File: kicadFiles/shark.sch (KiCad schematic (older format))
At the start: 258 parts, among them J1 USB_C_Receptacle, Q1 AO4406AL, SW1 MXSwitch, SW10 MXSwitch, SW11 MXSwitch, SW12 MXSwitch, SW13 MXSwitch, SW14 MXSwitch, SW15 MXSwitch, SW16 MXSwitch, SW17 MXSwitch, SW18 MXSwitch, SW19 MXSwitch, SW2 MXSwitch, SW20 MXSwitch, SW21 MXSwitch, SW22 MXSwitch, SW23 MXSwitch, SW24 MXSwitch, SW25 MXSwitch, SW26 MXSwitch, SW27 MXSwitch, SW28 MXSwitch, SW29 MXSwitch, SW3 MXSwitch, SW30 MXSwitch, SW31 MXSwitch, SW32 MXSwitch, SW33 MXSwitch, SW34 MXSwitch, SW35 MXSwitch, SW36 MXSwitch, SW37 MXSwitch, SW38 MXSwitch, SW39 MXSwitch, SW4 MXSwitch, SW40 MXSwitch, SW41 MXSwitch, SW42 MXSwitch, SW43 MXSwitch, SW44 MXSwitch, SW45 MXSwitch, SW46 MXSwitch, SW47 MXSwitch, SW48 MXSwitch, SW49 MXSwitch, SW5 MXSwitch, SW50 MXSwitch, SW51 MXSwitch, SW6 MXSwitch, SW7 MXSwitch, SW8 MXSwitch, SW9 MXSwitch, U1 STM32F303CCT7, U2 MCP1700-3302E_SOT23, Y1 8MHz

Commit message: Reorganized folders
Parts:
- D1, D48: footprint Keyboard_switches:D_SOD-123 -> acheronSymbols:D_SOD-123
- D10: renamed from D15; footprint Keyboard_switches:D_SOD-123 -> acheronSymbols:D_SOD-123
- D11: renamed from D27; footprint Keyboard_switches:D_SOD-123 -> acheronSymbols:D_SOD-123
- D12: renamed from D39; footprint Keyboard_switches:D_SOD-123 -> acheronSymbols:D_SOD-123
- D13: renamed from D4; footprint Keyboard_switches:D_SOD-123 -> acheronSymbols:D_SOD-123
- D14: renamed from D16; footprint Keyboard_switches:D_SOD-123 -> acheronSymbols:D_SOD-123
- D15: renamed from D28; footprint Keyboard_switches:D_SOD-123 -> acheronSymbols:D_SOD-123
- D16: renamed from D40; footprint Keyboard_switches:D_SOD-123 -> acheronSymbols:D_SOD-123
- D17: renamed from D5; footprint Keyboard_switches:D_SOD-123 -> acheronSymbols:D_SOD-123
- D18: renamed from D17; footprint Keyboard_switches:D_SOD-123 -> acheronSymbols:D_SOD-123
- D19: renamed from D29; footprint Keyboard_switches:D_SOD-123 -> acheronSymbols:D_SOD-123
- D2: renamed from D13; footprint Keyboard_switches:D_SOD-123 -> acheronSymbols:D_SOD-123
- D20: renamed from D41; footprint Keyboard_switches:D_SOD-123 -> acheronSymbols:D_SOD-123
- D21: renamed from D6; footprint Keyboard_switches:D_SOD-123 -> acheronSymbols:D_SOD-123
- D22: renamed from D18; footprint Keyboard_switches:D_SOD-123 -> acheronSymbols:D_SOD-123
- D23: renamed from D30; footprint Keyboard_switches:D_SOD-123 -> acheronSymbols:D_SOD-123
- D24: renamed from D42; footprint Keyboard_switches:D_SOD-123 -> acheronSymbols:D_SOD-123
- D25: renamed from D7; footprint Keyboard_switches:D_SOD-123 -> acheronSymbols:D_SOD-123
- D26: renamed from D19; footprint Keyboard_switches:D_SOD-123 -> acheronSymbols:D_SOD-123
- D27: renamed from D31; footprint Keyboard_switches:D_SOD-123 -> acheronSymbols:D_SOD-123
- D28: renamed from D43; footprint Keyboard_switches:D_SOD-123 -> acheronSymbols:D_SOD-123
- D29: renamed from D8; footprint Keyboard_switches:D_SOD-123 -> acheronSymbols:D_SOD-123
- D3: renamed from D25; footprint Keyboard_switches:D_SOD-123 -> acheronSymbols:D_SOD-123
- D30: renamed from D20; footprint Keyboard_switches:D_SOD-123 -> acheronSymbols:D_SOD-123
- D31: renamed from D32; footprint Keyboard_switches:D_SOD-123 -> acheronSymbols:D_SOD-123
- D32: renamed from D44; footprint Keyboard_switches:D_SOD-123 -> acheronSymbols:D_SOD-123
- D33: renamed from D9; footprint Keyboard_switches:D_SOD-123 -> acheronSymbols:D_SOD-123
- D34: renamed from D21; footprint Keyboard_switches:D_SOD-123 -> acheronSymbols:D_SOD-123
- D35: renamed from D33; footprint Keyboard_switches:D_SOD-123 -> acheronSymbols:D_SOD-123
- D36: renamed from D45; footprint Keyboard_switches:D_SOD-123 -> acheronSymbols:D_SOD-123
- D37: renamed from D10; footprint Keyboard_switches:D_SOD-123 -> acheronSymbols:D_SOD-123
- D38: renamed from D22; footprint Keyboard_switches:D_SOD-123 -> acheronSymbols:D_SOD-123
- D39: renamed from D34; footprint Keyboard_switches:D_SOD-123 -> acheronSymbols:D_SOD-123
- D4: renamed from D37; footprint Keyboard_switches:D_SOD-123 -> acheronSymbols:D_SOD-123
- D40: renamed from D46; footprint Keyboard_switches:D_SOD-123 -> acheronSymbols:D_SOD-123
- D41: renamed from D11; footprint Keyboard_switches:D_SOD-123 -> acheronSymbols:D_SOD-123
- D42: renamed from D23; footprint Keyboard_switches:D_SOD-123 -> acheronSymbols:D_SOD-123
- D43: renamed from D35; footprint Keyboard_switches:D_SOD-123 -> acheronSymbols:D_SOD-123
- D44: renamed from D47; footprint Keyboard_switches:D_SOD-123 -> acheronSymbols:D_SOD-123
- D45: renamed from D12; footprint Keyboard_switches:D_SOD-123 -> acheronSymbols:D_SOD-123
- D46: renamed from D24; footprint Keyboard_switches:D_SOD-123 -> acheronSymbols:D_SOD-123
- D47: renamed from D36; footprint Keyboard_switches:D_SOD-123 -> acheronSymbols:D_SOD-123
- D5: renamed from D2; footprint Keyboard_switches:D_SOD-123 -> acheronSymbols:D_SOD-123
- D6: renamed from D14; footprint Keyboard_switches:D_SOD-123 -> acheronSymbols:D_SOD-123
- D7: renamed from D26; footprint Keyboard_switches:D_SOD-123 -> acheronSymbols:D_SOD-123
- D8: renamed from D38; footprint Keyboard_switches:D_SOD-123 -> acheronSymbols:D_SOD-123
- D9: renamed from D3; footprint Keyboard_switches:D_SOD-123 -> acheronSymbols:D_SOD-123
- LED1, LED47: footprint Keyboard_switches:thtLED -> acheronSymbols:thtLED; symbol Keyboard_switches:LED -> acheronSymbols:LED
- LED10: renamed from LED15; footprint Keyboard_switches:thtLED -> acheronSymbols:thtLED; symbol Keyboard_switches:LED -> acheronSymbols:LED
- LED11: renamed from LED27; footprint Keyboard_switches:thtLED -> acheronSymbols:thtLED; symbol Keyboard_switches:LED -> acheronSymbols:LED
- LED12: renamed from LED39; footprint Keyboard_switches:thtLED -> acheronSymbols:thtLED; symbol Keyboard_switches:LED -> acheronSymbols:LED
- LED13: renamed from LED4; footprint Keyboard_switches:thtLED -> acheronSymbols:thtLED; symbol Keyboard_switches:LED -> acheronSymbols:LED
- LED14: renamed from LED16; footprint Keyboard_switches:thtLED -> acheronSymbols:thtLED; symbol Keyboard_switches:LED -> acheronSymbols:LED
- LED15: renamed from LED28; footprint Keyboard_switches:thtLED -> acheronSymbols:thtLED; symbol Keyboard_switches:LED -> acheronSymbols:LED
- LED16: renamed from LED40; footprint Keyboard_switches:thtLED -> acheronSymbols:thtLED; symbol Keyboard_switches:LED -> acheronSymbols:LED
- LED17: renamed from LED5; footprint Keyboard_switches:thtLED -> acheronSymbols:thtLED; symbol Keyboard_switches:LED -> acheronSymbols:LED
- LED18: renamed from LED17; footprint Keyboard_switches:thtLED -> acheronSymbols:thtLED; symbol Keyboard_switches:LED -> acheronSymbols:LED
- LED19: renamed from LED29; footprint Keyboard_switches:thtLED -> acheronSymbols:thtLED; symbol Keyboard_switches:LED -> acheronSymbols:LED
- LED2: renamed from LED13; footprint Keyboard_switches:thtLED -> acheronSymbols:thtLED; symbol Keyboard_switches:LED -> acheronSymbols:LED
- LED20: renamed from LED41; footprint Keyboard_switches:thtLED -> acheronSymbols:thtLED; symbol Keyboard_switches:LED -> acheronSymbols:LED
- LED21: renamed from LED49; footprint Keyboard_switches:thtLED -> acheronSymbols:thtLED; symbol Keyboard_switches:LED -> acheronSymbols:LED
- LED22: renamed from LED6; footprint Keyboard_switches:thtLED -> acheronSymbols:thtLED; symbol Keyboard_switches:LED -> acheronSymbols:LED
- LED23: renamed from LED18; footprint Keyboard_switches:thtLED -> acheronSymbols:thtLED; symbol Keyboard_switches:LED -> acheronSymbols:LED
- LED24: renamed from LED30; footprint Keyboard_switches:thtLED -> acheronSymbols:thtLED; symbol Keyboard_switches:LED -> acheronSymbols:LED
- LED25: renamed from LED42; footprint Keyboard_switches:thtLED -> acheronSymbols:thtLED; symbol Keyboard_switches:LED -> acheronSymbols:LED
- LED26: renamed from LED50; footprint Keyboard_switches:thtLED -> acheronSymbols:thtLED; symbol Keyboard_switches:LED -> acheronSymbols:LED
- LED27: renamed from LED7; footprint Keyboard_switches:thtLED -> acheronSymbols:thtLED; symbol Keyboard_switches:LED -> acheronSymbols:LED
- LED28: renamed from LED19; footprint Keyboard_switches:thtLED -> acheronSymbols:thtLED; symbol Keyboard_switches:LED -> acheronSymbols:LED
- LED29: renamed from LED31; footprint Keyboard_switches:thtLED -> acheronSymbols:thtLED; symbol Keyboard_switches:LED -> acheronSymbols:LED
- LED3: renamed from LED25; footprint Keyboard_switches:thtLED -> acheronSymbols:thtLED; symbol Keyboard_switches:LED -> acheronSymbols:LED
- LED30: renamed from LED43; footprint Keyboard_switches:thtLED -> acheronSymbols:thtLED; symbol Keyboard_switches:LED -> acheronSymbols:LED
- LED31: renamed from LED51; footprint Keyboard_switches:thtLED -> acheronSymbols:thtLED; symbol Keyboard_switches:LED -> acheronSymbols:LED
- LED32: renamed from LED8; footprint Keyboard_switches:thtLED -> acheronSymbols:thtLED; symbol Keyboard_switches:LED -> acheronSymbols:LED
- LED33: renamed from LED20; footprint Keyboard_switches:thtLED -> acheronSymbols:thtLED; symbol Keyboard_switches:LED -> acheronSymbols:LED
- LED34: renamed from LED32; footprint Keyboard_switches:thtLED -> acheronSymbols:thtLED; symbol Keyboard_switches:LED -> acheronSymbols:LED
- LED35: renamed from LED44; footprint Keyboard_switches:thtLED -> acheronSymbols:thtLED; symbol Keyboard_switches:LED -> acheronSymbols:LED
- LED36: renamed from LED9; footprint Keyboard_switches:thtLED -> acheronSymbols:thtLED; symbol Keyboard_switches:LED -> acheronSymbols:LED
- LED37: renamed from LED21; footprint Keyboard_switches:thtLED -> acheronSymbols:thtLED; symbol Keyboard_switches:LED -> acheronSymbols:LED
- LED38: renamed from LED33; footprint Keyboard_switches:thtLED -> acheronSymbols:thtLED; symbol Keyboard_switches:LED -> acheronSymbols:LED
- LED39: renamed from LED45; footprint Keyboard_switches:thtLED -> acheronSymbols:thtLED; symbol Keyboard_switches:LED -> acheronSymbols:LED
- LED4: renamed from LED37; footprint Keyboard_switches:thtLED -> acheronSymbols:thtLED; symbol Keyboard_switches:LED -> acheronSymbols:LED
- LED40: renamed from LED10; footprint Keyboard_switches:thtLED -> acheronSymbols:thtLED; symbol Keyboard_switches:LED -> acheronSymbols:LED
- LED41: renamed from LED22; footprint Keyboard_switches:thtLED -> acheronSymbols:thtLED; symbol Keyboard_switches:LED -> acheronSymbols:LED
- LED42: renamed from LED34; footprint Keyboard_switches:thtLED -> acheronSymbols:thtLED; symbol Keyboard_switches:LED -> acheronSymbols:LED
- LED43: renamed from LED46; footprint Keyboard_switches:thtLED -> acheronSymbols:thtLED; symbol Keyboard_switches:LED -> acheronSymbols:LED
- LED44: renamed from LED11; footprint Keyboard_switches:thtLED -> acheronSymbols:thtLED; symbol Keyboard_switches:LED -> acheronSymbols:LED
- LED45: renamed from LED23; footprint Keyboard_switches:thtLED -> acheronSymbols:thtLED; symbol Keyboard_switches:LED -> acheronSymbols:LED
- LED46: renamed from LED35; footprint Keyboard_switches:thtLED -> acheronSymbols:thtLED; symbol Keyboard_switches:LED -> acheronSymbols:LED
- LED48: renamed from LED12; footprint Keyboard_switches:thtLED -> acheronSymbols:thtLED; symbol Keyboard_switches:LED -> acheronSymbols:LED
- LED49: renamed from LED24; footprint Keyboard_switches:thtLED -> acheronSymbols:thtLED; symbol Keyboard_switches:LED -> acheronSymbols:LED
- LED5: renamed from LED2; footprint Keyboard_switches:thtLED -> acheronSymbols:thtLED; symbol Keyboard_switches:LED -> acheronSymbols:LED
- LED50: renamed from LED36; footprint Keyboard_switches:thtLED -> acheronSymbols:thtLED; symbol Keyboard_switches:LED -> acheronSymbols:LED
- LED51: renamed from LED48; footprint Keyboard_switches:thtLED -> acheronSymbols:thtLED; symbol Keyboard_switches:LED -> acheronSymbols:LED
- LED6: renamed from LED14; footprint Keyboard_switches:thtLED -> acheronSymbols:thtLED; symbol Keyboard_switches:LED -> acheronSymbols:LED
- LED7: renamed from LED26; footprint Keyboard_switches:thtLED -> acheronSymbols:thtLED; symbol Keyboard_switches:LED -> acheronSymbols:LED
- LED8: renamed from LED38; footprint Keyboard_switches:thtLED -> acheronSymbols:thtLED; symbol Keyboard_switches:LED -> acheronSymbols:LED
- LED9: renamed from LED3; footprint Keyboard_switches:thtLED -> acheronSymbols:thtLED; symbol Keyboard_switches:LED -> acheronSymbols:LED
- Q1: footprint Keyboard_switches:AO4406AL -> acheronSymbols:AO4406AL; symbol Keyboard_switches:AO4406AL -> acheronSymbols:AO4406AL
- RGB1, RGB8: footprint Keyboard_switches:LED_WS2812B -> acheronSymbols:LED_WS2812B
- RGB2: renamed from RGB5; footprint Keyboard_switches:LED_WS2812B -> acheronSymbols:LED_WS2812B
- RGB3: renamed from RGB2; footprint Keyboard_switches:LED_WS2812B -> acheronSymbols:LED_WS2812B
- RGB4: renamed from RGB6; footprint Keyboard_switches:LED_WS2812B -> acheronSymbols:LED_WS2812B
- RGB5: renamed from RGB3; footprint Keyboard_switches:LED_WS2812B -> acheronSymbols:LED_WS2812B
- RGB6: renamed from RGB7; footprint Keyboard_switches:LED_WS2812B -> acheronSymbols:LED_WS2812B
- RGB7: renamed from RGB4; footprint Keyboard_switches:LED_WS2812B -> acheronSymbols:LED_WS2812B
- SW1, SW47: footprint Keyboard_switches:MX100 -> acheronSymbols:MX100; symbol Keyboard_switches:MXSwitch -> acheronSymbols:MXSwitch
- SW10: renamed from SW15; footprint Keyboard_switches:MX100 -> acheronSymbols:MX100; symbol Keyboard_switches:MXSwitch -> acheronSymbols:MXSwitch
- SW11: renamed from SW27; footprint Keyboard_switches:MX100 -> acheronSymbols:MX100; symbol Keyboard_switches:MXSwitch -> acheronSymbols:MXSwitch
- SW12: renamed from SW39; footprint Keyboard_switches:MX100 -> acheronSymbols:MX100; symbol Keyboard_switches:MXSwitch -> acheronSymbols:MXSwitch
- SW13: renamed from SW4; footprint Keyboard_switches:MX100 -> acheronSymbols:MX100; symbol Keyboard_switches:MXSwitch -> acheronSymbols:MXSwitch
- SW14: renamed from SW16; footprint Keyboard_switches:MX100 -> acheronSymbols:MX100; symbol Keyboard_switches:MXSwitch -> acheronSymbols:MXSwitch
- SW15: renamed from SW28; footprint Keyboard_switches:MX100 -> acheronSymbols:MX100; symbol Keyboard_switches:MXSwitch -> acheronSymbols:MXSwitch
- SW16: renamed from SW40; footprint Keyboard_switches:MX100 -> acheronSymbols:MX100; symbol Keyboard_switches:MXSwitch -> acheronSymbols:MXSwitch
- SW17: renamed from SW5; footprint Keyboard_switches:MX100 -> acheronSymbols:MX100; symbol Keyboard_switches:MXSwitch -> acheronSymbols:MXSwitch
- SW18: renamed from SW17; footprint Keyboard_switches:MX100 -> acheronSymbols:MX100; symbol Keyboard_switches:MXSwitch -> acheronSymbols:MXSwitch
- SW19: renamed from SW29; footprint Keyboard_switches:MX100 -> acheronSymbols:MX100; symbol Keyboard_switches:MXSwitch -> acheronSymbols:MXSwitch
- SW2: renamed from SW13; footprint Keyboard_switches:MX100 -> acheronSymbols:MX100; symbol Keyboard_switches:MXSwitch -> acheronSymbols:MXSwitch
- SW20: renamed from SW41; footprint Keyboard_switches:MX100 -> acheronSymbols:MX100; symbol Keyboard_switches:MXSwitch -> acheronSymbols:MXSwitch
- SW21: renamed from SW49; footprint Keyboard_switches:MX200R -> acheronSymbols:MX200R; symbol Keyboard_switches:MXSwitch -> acheronSymbols:MXSwitch
- SW22: renamed from SW6; footprint Keyboard_switches:MX100 -> acheronSymbols:MX100; symbol Keyboard_switches:MXSwitch -> acheronSymbols:MXSwitch
- SW23: renamed from SW18; footprint Keyboard_switches:MX100 -> acheronSymbols:MX100; symbol Keyboard_switches:MXSwitch -> acheronSymbols:MXSwitch
- SW24: renamed from SW30; footprint Keyboard_switches:MX100 -> acheronSymbols:MX100; symbol Keyboard_switches:MXSwitch -> acheronSymbols:MXSwitch
- SW25: renamed from SW42; footprint Keyboard_switches:MX100 -> acheronSymbols:MX100; symbol Keyboard_switches:MXSwitch -> acheronSymbols:MXSwitch
- renumbered C9 to C1, C7 to C2, C1 to C3, C2 to C4, CSRT2 to CSRT1, H12 to H1, H1 to H2, H2 to H3, H3 to H4, H4 to H5, H5 to H6, H6 to H7, R6 to R1, R5 to R2, RA2 to RA1, RA1 to RA2, RB2 to RB1, RB1 to RB2, RL15 to RL10, RL27 to RL11, RL39 to RL12, RL4 to RL13, RL16 to RL14, RL28 to RL15, RL40 to RL16, RL5 to RL17, RL17 to RL18, RL29 to RL19, RL13 to RL2, RL41 to RL20, RL6 to RL21, RL18 to RL22, RL30 to RL23, RL42 to RL24, RL7 to RL25, RL19 to RL26, RL31 to RL27, RL43 to RL28, RL8 to RL29, RL25 to RL3, RL20 to RL30, RL32 to RL31, RL44 to RL32, RL9 to RL33, RL21 to RL34, RL33 to RL35, RL45 to RL36, RL10 to RL37, RL22 to RL38, RL34 to RL39, RL37 to RL4, RL46 to RL40, RL11 to RL41, RL23 to RL42, RL35 to RL43, RL47 to RL44, RL12 to RL45, RL24 to RL46, RL36 to RL47, RL2 to RL5, RL14 to RL6, RL26 to RL7, RL38 to RL8, RL3 to RL9, U2 to U1
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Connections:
- wire segments 620 -> 573

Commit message: Added encoder position and moved push button
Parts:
- added ROT2: Rotary_Encoder_Switch, acheronHardware:ALPS_EC11E, symbol Device:Rotary_Encoder_Switch
- D1, D48: footprint acheronSymbols:D_SOD-123 -> acheronComponents:D_SOD-123
- D10: renamed from D37; footprint acheronSymbols:D_SOD-123 -> acheronComponents:D_SOD-123
- D11: renamed from D41; footprint acheronSymbols:D_SOD-123 -> acheronComponents:D_SOD-123
- D12: renamed from D45; footprint acheronSymbols:D_SOD-123 -> acheronComponents:D_SOD-123
- D13: renamed from D2; footprint acheronSymbols:D_SOD-123 -> acheronComponents:D_SOD-123
- D14: renamed from D6; footprint acheronSymbols:D_SOD-123 -> acheronComponents:D_SOD-123
- D15: renamed from D10; footprint acheronSymbols:D_SOD-123 -> acheronComponents:D_SOD-123
- D16: renamed from D14; footprint acheronSymbols:D_SOD-123 -> acheronComponents:D_SOD-123
- D17: renamed from D18; footprint acheronSymbols:D_SOD-123 -> acheronComponents:D_SOD-123
- D18: renamed from D22; footprint acheronSymbols:D_SOD-123 -> acheronComponents:D_SOD-123
- D19: renamed from D26; footprint acheronSymbols:D_SOD-123 -> acheronComponents:D_SOD-123
- D2: renamed from D5; footprint acheronSymbols:D_SOD-123 -> acheronComponents:D_SOD-123
- D20: renamed from D30; footprint acheronSymbols:D_SOD-123 -> acheronComponents:D_SOD-123
- D21: renamed from D34; footprint acheronSymbols:D_SOD-123 -> acheronComponents:D_SOD-123
- D22: renamed from D38; footprint acheronSymbols:D_SOD-123 -> acheronComponents:D_SOD-123
- D23: renamed from D42; footprint acheronSymbols:D_SOD-123 -> acheronComponents:D_SOD-123
- D24: renamed from D46; footprint acheronSymbols:D_SOD-123 -> acheronComponents:D_SOD-123
- D25: renamed from D3; footprint acheronSymbols:D_SOD-123 -> acheronComponents:D_SOD-123
- D26: renamed from D7; footprint acheronSymbols:D_SOD-123 -> acheronComponents:D_SOD-123
- D27: renamed from D11; footprint acheronSymbols:D_SOD-123 -> acheronComponents:D_SOD-123
- D28: renamed from D15; footprint acheronSymbols:D_SOD-123 -> acheronComponents:D_SOD-123
- D29: renamed from D19; footprint acheronSymbols:D_SOD-123 -> acheronComponents:D_SOD-123
- D3: renamed from D9; footprint acheronSymbols:D_SOD-123 -> acheronComponents:D_SOD-123
- D30: renamed from D23; footprint acheronSymbols:D_SOD-123 -> acheronComponents:D_SOD-123
- D31: renamed from D27; footprint acheronSymbols:D_SOD-123 -> acheronComponents:D_SOD-123
- D32: renamed from D31; footprint acheronSymbols:D_SOD-123 -> acheronComponents:D_SOD-123
- D33: renamed from D35; footprint acheronSymbols:D_SOD-123 -> acheronComponents:D_SOD-123
- D34: renamed from D39; footprint acheronSymbols:D_SOD-123 -> acheronComponents:D_SOD-123
- D35: renamed from D43; footprint acheronSymbols:D_SOD-123 -> acheronComponents:D_SOD-123
- D36: renamed from D47; footprint acheronSymbols:D_SOD-123 -> acheronComponents:D_SOD-123
- D37: renamed from D4; footprint acheronSymbols:D_SOD-123 -> acheronComponents:D_SOD-123
- D38: renamed from D8; footprint acheronSymbols:D_SOD-123 -> acheronComponents:D_SOD-123
- D39: renamed from D12; footprint acheronSymbols:D_SOD-123 -> acheronComponents:D_SOD-123
- D4: renamed from D13; footprint acheronSymbols:D_SOD-123 -> acheronComponents:D_SOD-123
- D40: renamed from D16; footprint acheronSymbols:D_SOD-123 -> acheronComponents:D_SOD-123
- D41: renamed from D20; footprint acheronSymbols:D_SOD-123 -> acheronComponents:D_SOD-123
- D42: renamed from D24; footprint acheronSymbols:D_SOD-123 -> acheronComponents:D_SOD-123
- D43: renamed from D28; footprint acheronSymbols:D_SOD-123 -> acheronComponents:D_SOD-123
- D44: renamed from D32; footprint acheronSymbols:D_SOD-123 -> acheronComponents:D_SOD-123
- D45: renamed from D36; footprint acheronSymbols:D_SOD-123 -> acheronComponents:D_SOD-123
- D46: renamed from D40; footprint acheronSymbols:D_SOD-123 -> acheronComponents:D_SOD-123
- D47: renamed from D44; footprint acheronSymbols:D_SOD-123 -> acheronComponents:D_SOD-123
- D5: renamed from D17; footprint acheronSymbols:D_SOD-123 -> acheronComponents:D_SOD-123
- D6: renamed from D21; footprint acheronSymbols:D_SOD-123 -> acheronComponents:D_SOD-123
- D7: renamed from D25; footprint acheronSymbols:D_SOD-123 -> acheronComponents:D_SOD-123
- D8: renamed from D29; footprint acheronSymbols:D_SOD-123 -> acheronComponents:D_SOD-123
- D9: renamed from D33; footprint acheronSymbols:D_SOD-123 -> acheronComponents:D_SOD-123
- DF1: footprint Diode_SMD:D_SOD-123 -> acheronComponents:D_SOD-123
- LED1, LED47: footprint acheronSymbols:thtLED -> acheronComponents:thtLED
- LED10: renamed from LED40; footprint acheronSymbols:thtLED -> acheronComponents:thtLED
- LED11: renamed from LED44; footprint acheronSymbols:thtLED -> acheronComponents:thtLED
- LED12: renamed from LED48; footprint acheronSymbols:thtLED -> acheronComponents:thtLED
- LED13: renamed from LED2; footprint acheronSymbols:thtLED -> acheronComponents:thtLED
- LED14: renamed from LED6; footprint acheronSymbols:thtLED -> acheronComponents:thtLED
- LED15: renamed from LED10; footprint acheronSymbols:thtLED -> acheronComponents:thtLED
- LED16: renamed from LED14; footprint acheronSymbols:thtLED -> acheronComponents:thtLED
- LED17: renamed from LED18; footprint acheronSymbols:thtLED -> acheronComponents:thtLED
- LED18: renamed from LED23; footprint acheronSymbols:thtLED -> acheronComponents:thtLED
- LED19: renamed from LED28; footprint acheronSymbols:thtLED -> acheronComponents:thtLED
- LED2: renamed from LED5; footprint acheronSymbols:thtLED -> acheronComponents:thtLED
- LED20: renamed from LED33; footprint acheronSymbols:thtLED -> acheronComponents:thtLED
- LED21: renamed from LED37; footprint acheronSymbols:thtLED -> acheronComponents:thtLED
- LED22: renamed from LED41; footprint acheronSymbols:thtLED -> acheronComponents:thtLED
- LED23: renamed from LED45; footprint acheronSymbols:thtLED -> acheronComponents:thtLED
- LED24: renamed from LED49; footprint acheronSymbols:thtLED -> acheronComponents:thtLED
- LED25: renamed from LED3; footprint acheronSymbols:thtLED -> acheronComponents:thtLED
- LED26: renamed from LED7; footprint acheronSymbols:thtLED -> acheronComponents:thtLED
- LED27: renamed from LED11; footprint acheronSymbols:thtLED -> acheronComponents:thtLED
- LED28: renamed from LED15; footprint acheronSymbols:thtLED -> acheronComponents:thtLED
- LED29: renamed from LED19; footprint acheronSymbols:thtLED -> acheronComponents:thtLED
- LED3: renamed from LED9; footprint acheronSymbols:thtLED -> acheronComponents:thtLED
- LED30: renamed from LED24; footprint acheronSymbols:thtLED -> acheronComponents:thtLED
- LED31: renamed from LED29; footprint acheronSymbols:thtLED -> acheronComponents:thtLED
- LED32: renamed from LED34; footprint acheronSymbols:thtLED -> acheronComponents:thtLED
- LED33: renamed from LED38; footprint acheronSymbols:thtLED -> acheronComponents:thtLED
- LED34: renamed from LED42; footprint acheronSymbols:thtLED -> acheronComponents:thtLED
- LED35: renamed from LED46; footprint acheronSymbols:thtLED -> acheronComponents:thtLED
- LED36: renamed from LED50; footprint acheronSymbols:thtLED -> acheronComponents:thtLED
- LED37: renamed from LED4; footprint acheronSymbols:thtLED -> acheronComponents:thtLED
- LED38: renamed from LED8; footprint acheronSymbols:thtLED -> acheronComponents:thtLED
- LED39: renamed from LED12; footprint acheronSymbols:thtLED -> acheronComponents:thtLED
- LED4: renamed from LED13; footprint acheronSymbols:thtLED -> acheronComponents:thtLED
- LED40: renamed from LED16; footprint acheronSymbols:thtLED -> acheronComponents:thtLED
- LED41: renamed from LED20; footprint acheronSymbols:thtLED -> acheronComponents:thtLED
- LED42: renamed from LED25; footprint acheronSymbols:thtLED -> acheronComponents:thtLED
- LED43: renamed from LED30; footprint acheronSymbols:thtLED -> acheronComponents:thtLED
- LED44: renamed from LED35; footprint acheronSymbols:thtLED -> acheronComponents:thtLED
- LED45: renamed from LED39; footprint acheronSymbols:thtLED -> acheronComponents:thtLED
- LED46: renamed from LED43; footprint acheronSymbols:thtLED -> acheronComponents:thtLED
- LED48: renamed from LED51; footprint acheronSymbols:thtLED -> acheronComponents:thtLED
- LED49: renamed from LED21; footprint acheronSymbols:thtLED -> acheronComponents:thtLED
- LED5: renamed from LED17; footprint acheronSymbols:thtLED -> acheronComponents:thtLED
- LED50: renamed from LED26; footprint acheronSymbols:thtLED -> acheronComponents:thtLED
- LED51: renamed from LED31; footprint acheronSymbols:thtLED -> acheronComponents:thtLED
- LED6: renamed from LED22; footprint acheronSymbols:thtLED -> acheronComponents:thtLED
- LED7: renamed from LED27; footprint acheronSymbols:thtLED -> acheronComponents:thtLED
- LED8: renamed from LED32; footprint acheronSymbols:thtLED -> acheronComponents:thtLED
- LED9: renamed from LED36; footprint acheronSymbols:thtLED -> acheronComponents:thtLED
- Q1: footprint acheronSymbols:AO4406AL -> acheronComponents:AO4406AL
- RGB1, RGB8: footprint acheronSymbols:LED_WS2812B -> acheronComponents:LED_WS2812B
- RGB2: renamed from RGB3; footprint acheronSymbols:LED_WS2812B -> acheronComponents:LED_WS2812B
- RGB3: renamed from RGB5; footprint acheronSymbols:LED_WS2812B -> acheronComponents:LED_WS2812B
- RGB4: renamed from RGB7; footprint acheronSymbols:LED_WS2812B -> acheronComponents:LED_WS2812B
- RGB5: renamed from RGB2; footprint acheronSymbols:LED_WS2812B -> acheronComponents:LED_WS2812B
- RGB6: renamed from RGB4; footprint acheronSymbols:LED_WS2812B -> acheronComponents:LED_WS2812B
- RGB7: renamed from RGB6; footprint acheronSymbols:LED_WS2812B -> acheronComponents:LED_WS2812B
- ROT1: footprint encoders:ALPS_EC11E -> acheronHardware:ALPS_EC11E
- SW1, SW47: footprint acheronSymbols:MX100 -> acheronKeyboardSwitches:MX100
- SW10: renamed from SW40; footprint acheronSymbols:MX100 -> acheronKeyboardSwitches:MX100
- SW11: renamed from SW44; footprint acheronSymbols:MX100 -> acheronKeyboardSwitches:MX100
- SW12: renamed from SW48; footprint acheronSymbols:MX100 -> acheronKeyboardSwitches:MX100
- SW13: renamed from SW2; footprint acheronSymbols:MX100 -> acheronKeyboardSwitches:MX100
- SW14: renamed from SW6; footprint acheronSymbols:MX100 -> acheronKeyboardSwitches:MX100
- SW15: renamed from SW10; footprint acheronSymbols:MX100 -> acheronKeyboardSwitches:MX100
- SW16: renamed from SW14; footprint acheronSymbols:MX100 -> acheronKeyboardSwitches:MX100
- SW17: renamed from SW18; footprint acheronSymbols:MX100 -> acheronKeyboardSwitches:MX100
- SW18: renamed from SW23; footprint acheronSymbols:MX100 -> acheronKeyboardSwitches:MX100
- SW19: renamed from SW28; footprint acheronSymbols:MX100 -> acheronKeyboardSwitches:MX100
- SW2: renamed from SW5; footprint acheronSymbols:MX100 -> acheronKeyboardSwitches:MX100
- SW20: renamed from SW33; footprint acheronSymbols:MX100 -> acheronKeyboardSwitches:MX100
- SW21: renamed from SW37; footprint acheronSymbols:MX100 -> acheronKeyboardSwitches:MX100
- SW22: renamed from SW41; footprint acheronSymbols:MX100 -> acheronKeyboardSwitches:MX100
- SW23: renamed from SW45; footprint acheronSymbols:MX100 -> acheronKeyboardSwitches:MX100
- SW24: renamed from SW49; footprint acheronSymbols:MX100 -> acheronKeyboardSwitches:MX100
- SW25: renamed from SW3; footprint acheronSymbols:MX100 -> acheronKeyboardSwitches:MX100
- SW26: renamed from SW7; footprint acheronSymbols:MX100 -> acheronKeyboardSwitches:MX100
- SW27: renamed from SW11; footprint acheronSymbols:MX100 -> acheronKeyboardSwitches:MX100
- SW28: renamed from SW15; footprint acheronSymbols:MX100 -> acheronKeyboardSwitches:MX100
- SW29: renamed from SW19; footprint acheronSymbols:MX100 -> acheronKeyboardSwitches:MX100
- SW3: renamed from SW9; footprint acheronSymbols:MX100 -> acheronKeyboardSwitches:MX100
- SW30: renamed from SW24; footprint acheronSymbols:MX100 -> acheronKeyboardSwitches:MX100
- SW31: renamed from SW29; footprint acheronSymbols:MX100 -> acheronKeyboardSwitches:MX100
- SW32: renamed from SW34; footprint acheronSymbols:MX100 -> acheronKeyboardSwitches:MX100
- SW33: renamed from SW38; footprint acheronSymbols:MX100 -> acheronKeyboardSwitches:MX100
- SW34: renamed from SW42; footprint acheronSymbols:MX100 -> acheronKeyboardSwitches:MX100
- SW35: renamed from SW46; footprint acheronSymbols:MX100 -> acheronKeyboardSwitches:MX100
- SW36: renamed from SW50; footprint acheronSymbols:MX100 -> acheronKeyboardSwitches:MX100
- SW37: renamed from SW4; footprint acheronSymbols:MX100 -> acheronKeyboardSwitches:MX100
- SW38: renamed from SW8; footprint acheronSymbols:MX100 -> acheronKeyboardSwitches:MX100
- SW39: renamed from SW12; footprint acheronSymbols:MX100 -> acheronKeyboardSwitches:MX100
- SW4: renamed from SW13; footprint acheronSymbols:MX100 -> acheronKeyboardSwitches:MX100
- SW40: renamed from SW16; footprint acheronSymbols:MX100 -> acheronKeyboardSwitches:MX100
- SW41: renamed from SW20; footprint acheronSymbols:MX100 -> acheronKeyboardSwitches:MX100
- SW42: renamed from SW25; footprint acheronSymbols:MX100 -> acheronKeyboardSwitches:MX100
- SW43: renamed from SW30; footprint acheronSymbols:MX100 -> acheronKeyboardSwitches:MX100
- SW44: renamed from SW35; footprint acheronSymbols:MX100 -> acheronKeyboardSwitches:MX100
- SW45: renamed from SW39; footprint acheronSymbols:MX100 -> acheronKeyboardSwitches:MX100
- SW46: renamed from SW43; footprint acheronSymbols:MX100 -> acheronKeyboardSwitches:MX100
- SW48: renamed from SW51; footprint acheronSymbols:MX100 -> acheronKeyboardSwitches:MX100
- SW49: renamed from SW21; footprint acheronSymbols:MX200R -> acheronKeyboardSwitches:MX200R
- SW5: renamed from SW17; footprint acheronSymbols:MX100 -> acheronKeyboardSwitches:MX100
- SW50: renamed from SW26; footprint acheronSymbols:MX200R -> acheronKeyboardSwitches:MX200R
- SW51: renamed from SW31; footprint acheronSymbols:MX200R -> acheronKeyboardSwitches:MX200R
- SW6: renamed from SW22; footprint acheronSymbols:MX100 -> acheronKeyboardSwitches:MX100
- SW7: renamed from SW27; footprint acheronSymbols:MX100 -> acheronKeyboardSwitches:MX100
- renumbered C3 to C1, C4 to C2, C2 to C7, C1 to C9, CSRT1 to CRST2, H2 to H1, H3 to H2, H4 to H3, H5 to H4, H6 to H5, H7 to H6, H1 to H7, R2 to R5, R1 to R6, RA2 to RA1, RA1 to RA2, RB2 to RB1, RB1 to RB2, RL37 to RL10, RL41 to RL11, RL45 to RL12, RL2 to RL13, RL6 to RL14, RL10 to RL15, RL14 to RL16, RL18 to RL17, RL22 to RL18, RL26 to RL19, RL5 to RL2, RL30 to RL20, RL34 to RL21, RL38 to RL22, RL42 to RL23, RL46 to RL24, RL3 to RL25, RL7 to RL26, RL11 to RL27, RL15 to RL28, RL19 to RL29, RL9 to RL3, RL23 to RL30, RL27 to RL31, RL31 to RL32, RL35 to RL33, RL39 to RL34, RL43 to RL35, RL47 to RL36, RL4 to RL37, RL8 to RL38, RL12 to RL39, RL13 to RL4, RL16 to RL40, RL20 to RL41, RL24 to RL42, RL28 to RL43, RL32 to RL44, RL36 to RL45, RL40 to RL46, RL44 to RL47, RL17 to RL5, RL21 to RL6, RL25 to RL7, RL29 to RL8, RL33 to RL9, U2 to U1, U1 to U2
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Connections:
- net Col12: now also ROT2.S2
- net EncA: now also ROT2.A
- net EncB: now also ROT2.B
- net GND: now also ROT2.C
- net EncS3: now reaches D48.2 (A), SW48.2 (Row)
- net EncS3: now also ROT2.S1
- net at LED1.K, LED13.K, LED25.K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: now also LED10.K, LED11.K, LED12.K, LED14.K, LED15.K, LED16.K, LED17.K, LED18.K, LED19.K, LED2.K, LED20.K, LED21.K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
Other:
- note added: "ESD\nProtection"
- note added: "Logos and flags"
- note added: "MCU and crystal"
- note added: "Mounting holes"
- note added: "RGB"
- note added: "Switch LED matrix"
- note added: "Switch matrix\n"
- note added: "USB Connector"
- note added: "Voltage regulation\ncapacitor bank\n"
- note removed: "ESD Protection"
- note removed: "Voltage regulation capacitor bank\n"
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
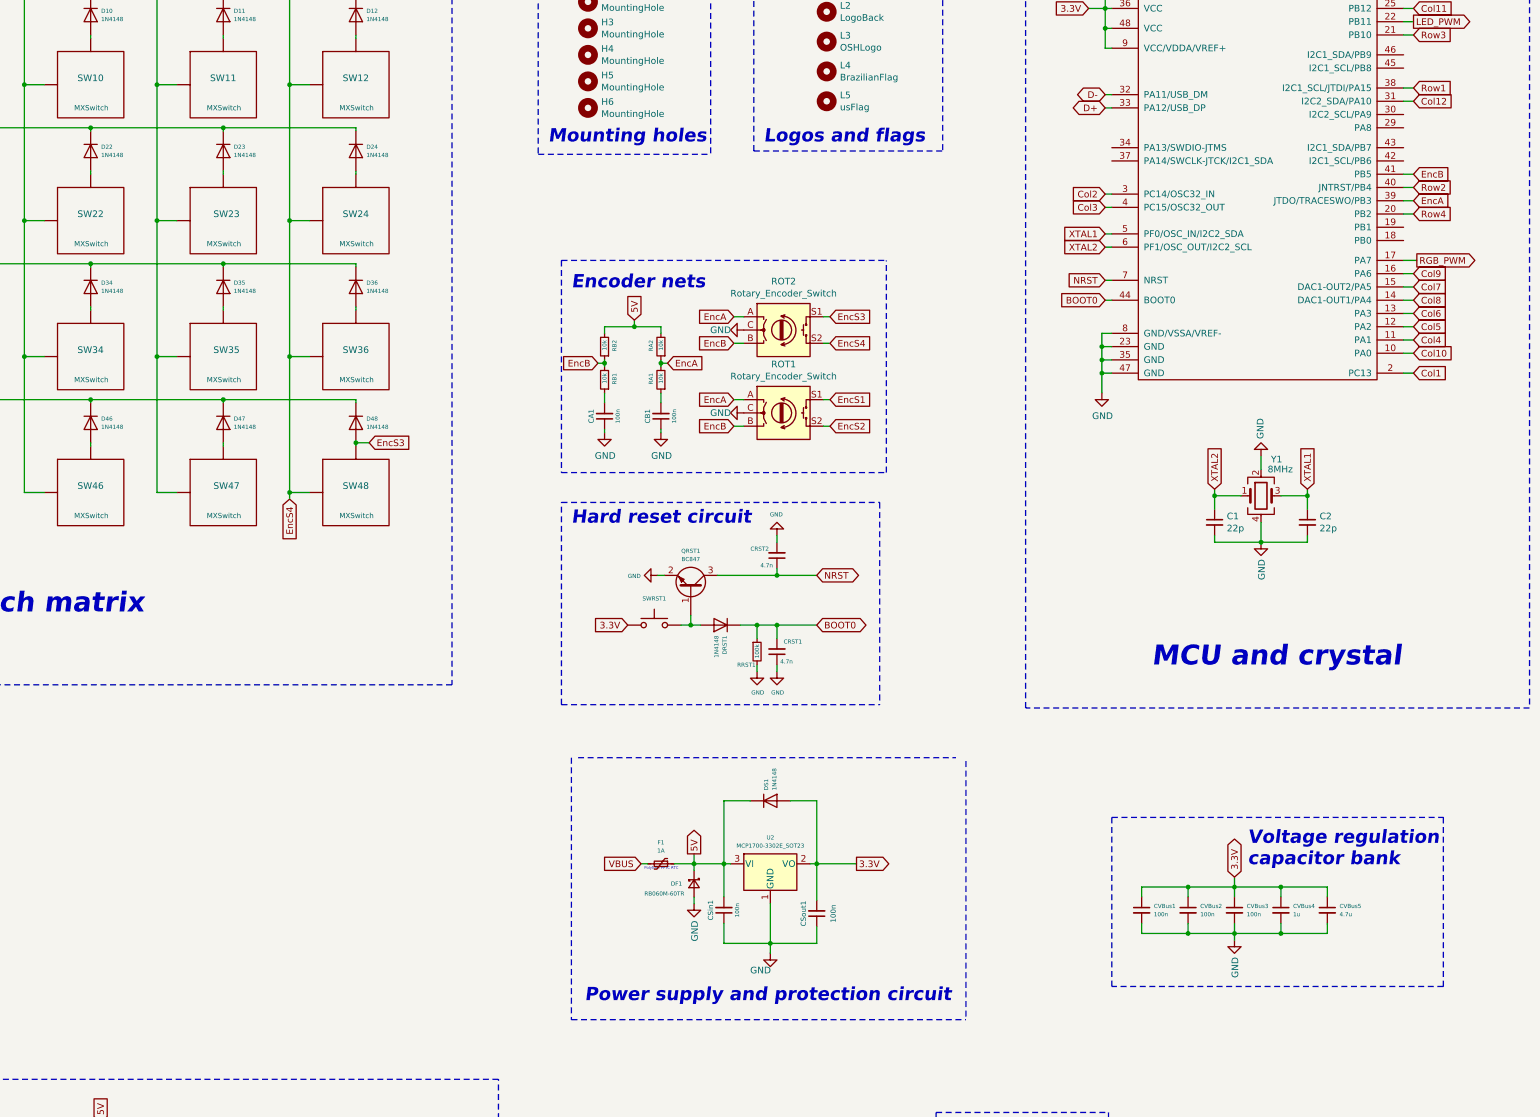
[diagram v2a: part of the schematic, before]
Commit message: Added I2C pins and hi-pro compatible plates
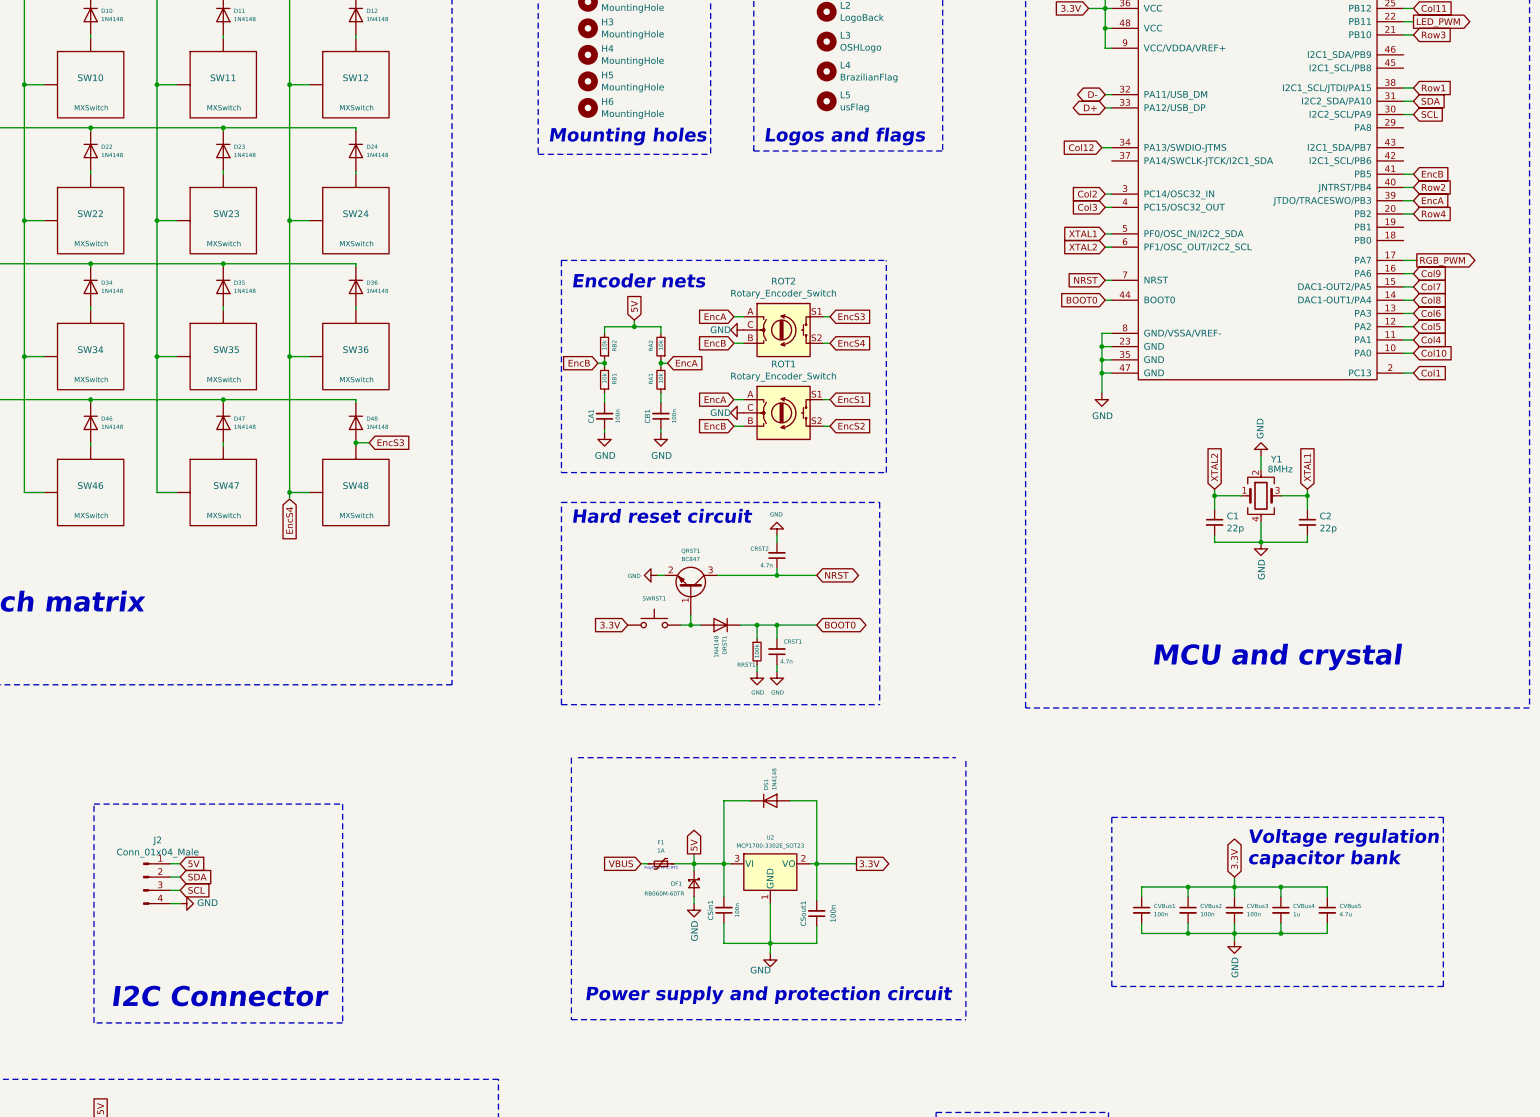
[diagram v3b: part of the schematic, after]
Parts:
- added J2: Conn_01x04_Male, acheronConnectors:JSTBM04B-ASRS, symbol Connector:Conn_01x04_Male
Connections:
- net 5V: now also J2.1 (Pin_1)
- net Col12: now also U1.34 (PA13/SWDIO-JTMS); no longer U1.31 (I2C2_SDA/PA10)
- net GND: now also J2.4 (Pin_4)
- net SCL: now reaches U1.30 (I2C2_SCL/PA9)
- net SCL: now also J2.3 (Pin_3)
- new net SDA: J2.2 (Pin_2), U1.31 (I2C2_SDA/PA10)
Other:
- note added: "I2C Connector"
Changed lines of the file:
@@
 Sheet 1 1
 Title "SharkPCB"
-Date "2019-03-12"
-Rev "Rev 3.1.2"
+Date "2019-03-13"
+Rev "Rev 3.1.3"
 Comp "Gondolin Electronics"
 Comment1 ""
@@
 	1    0    0    -1
 $EndComp
-Text GLabel 21450 4100 2    50   Input ~ 0
+Text GLabel 19100 4450 0    50   Input ~ 0
 Col12
-Wire Wire Line
-	21450 4100 21375 4100
 Text GLabel 19125 4800 0    50   Input ~ 0
 Col2
@@
 Wire Wire Line
 	4525 10700 4800 10700
+$Comp
+L Connector:Conn_01x04_Male J2
+U 1 1 5C8FE384
+P 11875 9950
+F 0 "J2" H 11981 10228 50  0000 C CNN
+F 1 "Conn_01x04_Male" H 11981 10137 50  0000 C CNN
+F 2 "acheronConnectors:JSTBM04B-ASRS" H 11875 9950 50  0001 C CNN
+F 3 "~" H 11875 9950 50  0001 C CNN
+	1    11875 9950
+	1    0    0    -1
+$EndComp
+Wire Wire Line
+	12075 9850 12150 9850
+Text GLabel 12150 9850 2    50   Input ~ 0
+5V
+Wire Wire Line
+	12075 10150 12150 10150
+$Comp
+L power:GND #PWR0102
+U 1 1 5C9D3CEB
+P 12150 10150
+F 0 "#PWR0102" H 12150 9900 50  0001 C CNN
+F 1 "GND" V 12155 10022 50  0000 R CNN
+F 2 "" H 12150 10150 50  0001 C CNN
+F 3 "" H 12150 10150 50  0001 C CNN
+	1    12150 10150
+	0    -1   -1   0
+$EndComp
+Wire Wire Line
+	12075 9950 12150 9950
+Text GLabel 12150 9950 2    50   Input ~ 0
+SDA
+Text GLabel 12150 10050 2    50   Input ~ 0
+SCL
+Wire Wire Line
+	12150 10050 12075 10050
+Wire Notes Line width 20
+	11500 9400 13375 9400
+Wire Notes Line width 20
+	13375 9400 13375 11050
+Wire Notes Line width 20
+	13375 11050 11500 11050
+Wire Notes Line width 20
+	11500 11050 11500 9400
+Text Notes 11625 10950 0    150  Italic 30
+I2C Connector
+Text GLabel 21450 4200 2    50   Input ~ 0
+SCL
+Text GLabel 21450 4100 2    50   Input ~ 0
+SDA
+Wire Wire Line
+	21450 4200 21375 4200
+Wire Wire Line
+	21375 4100 21450 4100
+Wire Wire Line
+	19100 4450 19175 4450
 $EndSCHEMATC

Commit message: [Feature] Changed the I2C pins to a common pin header
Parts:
- J2: footprint acheronConnectors:JSTBM04B-ASRS -> acheronConnectors:4pinHeader
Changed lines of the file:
@@
 F 0 "J2" H 11981 10228 50  0000 C CNN
 F 1 "Conn_01x04_Male" H 11981 10137 50  0000 C CNN
-F 2 "acheronConnectors:JSTBM04B-ASRS" H 11875 9950 50  0001 C CNN
+F 2 "acheronConnectors:4pinHeader" H 11875 9950 50  0001 C CNN
 F 3 "~" H 11875 9950 50  0001 C CNN
 	1    11875 9950
